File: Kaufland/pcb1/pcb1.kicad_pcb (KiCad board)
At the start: 2 copper layers, 118.4 x 66.5 mm, 15 parts, among them J1 AudioJack2, J2 Barrel_Jack, SW1 SW_Push, U1 DF_Player, U2 RGB_LED_STRIP

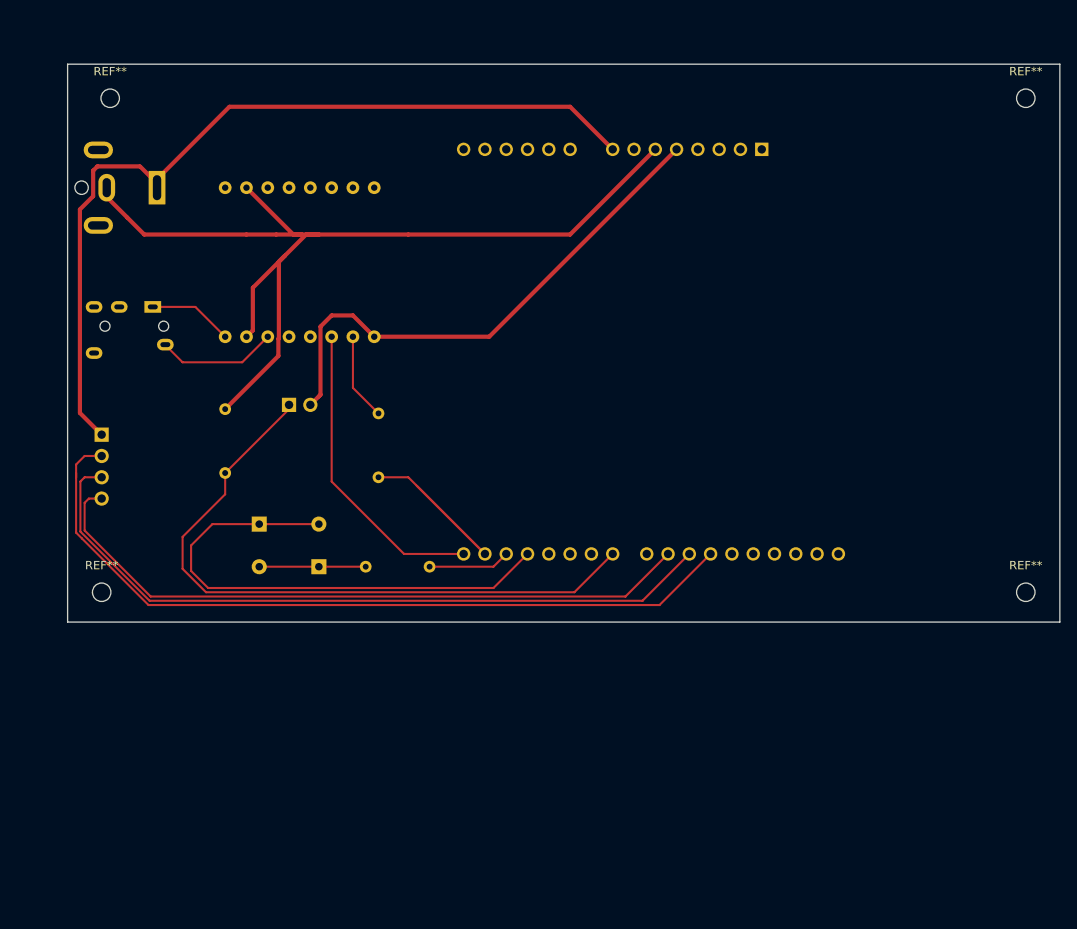
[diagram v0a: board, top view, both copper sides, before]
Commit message: finished pcb v1.0
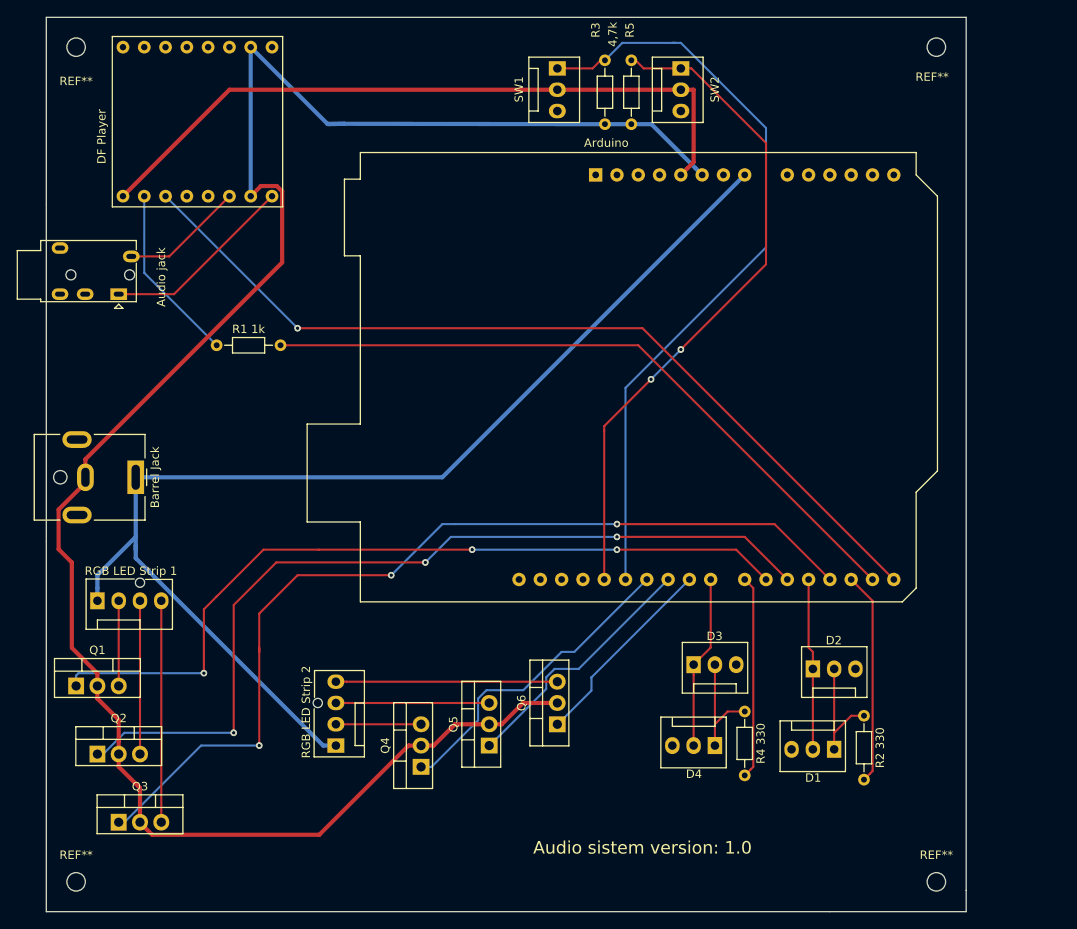
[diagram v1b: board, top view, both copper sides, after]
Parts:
- removed A1: Arduino_UNO_R3, Module:Arduino_UNO_R3
- removed J1: AudioJack2, Connector_Audio:Jack_3.5mm_PJ320E_Horizontal
- removed J2: Barrel_Jack, Connector_BarrelJack:BarrelJack_CUI_PJ-063AH_Horizontal
- removed R1: 1k, Resistor_THT:R_Axial_DIN0204_L3.6mm_D1.6mm_P7.62mm_Horizontal
- removed R2: 330, Resistor_THT:R_Axial_DIN0204_L3.6mm_D1.6mm_P7.62mm_Horizontal
- removed the REF** at (164.1, 54.4)
- removed the REF** at (164.1, 113.3)
- removed the REF** at (53.8, 113.3)
- removed the REF** at (54.9, 54.4)
- removed U1: DF_Player, pcb1:DFPlayerMini
- removed U2: RGB_LED_STRIP, Connector_PinHeader_2.54mm:PinHeader_1x04_P2.54mm_Vertical
- added Arduino: Arduino_UNO_R3, Module:Arduino_UNO_R3, F.Cu at (112.8, 63.5)
- added Audio jack: AudioJack2, Connector_Audio:Jack_3.5mm_PJ320E_Horizontal, F.Cu at (55.9, 77.7)
- added Barrel Jack: Barrel_Jack, Connector_BarrelJack:BarrelJack_CUI_PJ-063AH_Horizontal, F.Cu at (57.9, 99.6)
- added D3: LED, Connector:FanPinHeader_1x03_P2.54mm_Vertical, F.Cu at (124.5, 121.9)
- added D4: LED, Connector:FanPinHeader_1x03_P2.54mm_Vertical, F.Cu at (127.0, 131.6)
- added DF Player: DF_Player, pcb1:DFPlayerMini, F.Cu at (66.5, 58.4)
- added Q1: IRLB8721PBF, Package_TO_SOT_THT:TO-220-3_Vertical, F.Cu at (50.8, 124.5)
- added Q2: IRLB8721PBF, Package_TO_SOT_THT:TO-220-3_Vertical, F.Cu at (53.3, 132.6)
- added Q3: IRLB8721PBF, Package_TO_SOT_THT:TO-220-3_Vertical, F.Cu at (55.9, 140.7)
- added Q4: IRLB8721PBF, Package_TO_SOT_THT:TO-220-3_Vertical, F.Cu at (91.9, 134.1)
- added Q5: IRLB8721PBF, Package_TO_SOT_THT:TO-220-3_Vertical, F.Cu at (100.1, 131.6)
- added Q6: IRLB8721PBF, Package_TO_SOT_THT:TO-220-3_Vertical, F.Cu at (108.2, 129.0)
- added R1 1k: 1k, Resistor_THT:R_Axial_DIN0204_L3.6mm_D1.6mm_P7.62mm_Horizontal, F.Cu at (67.6, 83.8)
- added R2 330: 330, Resistor_THT:R_Axial_DIN0204_L3.6mm_D1.6mm_P7.62mm_Horizontal, F.Cu at (144.8, 128.0)
- added R4 330: 330, Resistor_THT:R_Axial_DIN0204_L3.6mm_D1.6mm_P7.62mm_Horizontal, F.Cu at (130.6, 127.5)
- added R5: 4.7k, Resistor_THT:R_Axial_DIN0204_L3.6mm_D1.6mm_P7.62mm_Horizontal, F.Cu at (117.0, 49.8)
- added REF**: MountingHole_2.2mm_M2, MountingHole:MountingHole_2.2mm_M2, F.Cu at (50.8, 48.3)
- added REF**: MountingHole_2.2mm_M2, MountingHole:MountingHole_2.2mm_M2, F.Cu at (153.4, 48.3)
- added REF**: MountingHole_2.2mm_M2, MountingHole:MountingHole_2.2mm_M2, F.Cu at (153.4, 147.8)
- added REF**: MountingHole_2.2mm_M2, MountingHole:MountingHole_2.2mm_M2, F.Cu at (50.8, 147.8)
- added RGB LED Strip 1: RGB_LED_STRIP-My_Library, Connector:FanPinHeader_1x04_P2.54mm_Vertical, F.Cu at (53.3, 114.3)
- added RGB LED Strip 2: RGB_LED_STRIP-My_Library, Connector:FanPinHeader_1x04_P2.54mm_Vertical, F.Cu at (81.8, 131.6)
- added SW2: SW_Push, Connector:FanPinHeader_1x03_P2.54mm_Vertical, F.Cu at (122.9, 50.8)
- D1, D2: footprint Diode_THT:D_A-405_P5.08mm_Vertical_KathodeUp -> Connector:FanPinHeader_1x03_P2.54mm_Vertical; moved to F.Cu
- R3: moved to F.Cu
- SW1: footprint Connector_PinHeader_2.54mm:PinHeader_1x02_P2.54mm_Vertical -> Connector:FanPinHeader_1x03_P2.54mm_Vertical; moved to F.Cu
- moved D2 68.3 mm to (138.7, 122.4), turned to 0 degrees
- moved R3 66.9 mm to (113.9, 49.8), turned to 270 degrees
- moved D1 65.2 mm to (141.2, 132.0), turned to 180 degrees
- moved SW1 51.3 mm to (108.2, 50.8)
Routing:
- net GNDREF: track 118.4 -> 231.7 mm
- net Net-(A1-Pad18): track 0.00 -> 112.0 mm, vias 0 -> 3
- net Net-(A1-Pad20): track 0.00 -> 104.1 mm, vias 0 -> 3
- net Net-(A1-Pad21): track 0.00 -> 95.7 mm, vias 0 -> 3
- net Net-(A1-Pad28): track 0.00 -> 80.6 mm, vias 0 -> 2
- net Net-(A1-Pad15): track 36.6 -> 105.8 mm, vias 0 -> 1
- net Net-(A1-Pad25): track 87.1 -> 30.4 mm
- net Net-(A1-Pad24): track 80.5 -> 23.8 mm
- net Net-(A1-Pad26): track 93.9 -> 37.7 mm
- net Net-(A1-Pad16): track 28.0 -> 82.2 mm
- net Net-(A1-Pad19): track 62.0 -> 21.2 mm
- net +12V: track 103.0 -> 140.4 mm
- net Net-(Q3-Pad3): track 0.00 -> 26.4 mm
- net Net-(Q6-Pad3): track 0.00 -> 26.4 mm
- net Net-(A1-Pad22): track 0.00 -> 24.2 mm
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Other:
- board size 118.4 x 66.5 mm -> 109.7 x 106.7 mm
- board text added: "4,7k"
- board text added: "Audio sistem version: 1.0"
